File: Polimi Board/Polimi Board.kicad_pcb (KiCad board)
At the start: 2 copper layers, 96 parts, among them IC1 M95512-RMN6P, J1 I2C Oled Screen, J2 DM3AT-SF-PEJM5_40_, J3 65100516121, J4 UART Conn, J5 JTAG Conn, J7 65100516121, J8 7499010121A, SW1 MCU Reset, SW2 SW_Push, SW3 SW_Push, SW4 SW_Push, SW5 SW_Push, SW6 SW_Push, SW7 SW_Push, SW8 SW_Push, U1 STM32F205RCT6, U2 FT2232HL, U3 LAN8742A, U5 TLV76133DCY, Y1 ABL-25.000MHz-B1UB, Y2 ABL-12.000MHZ-20-D4HFI

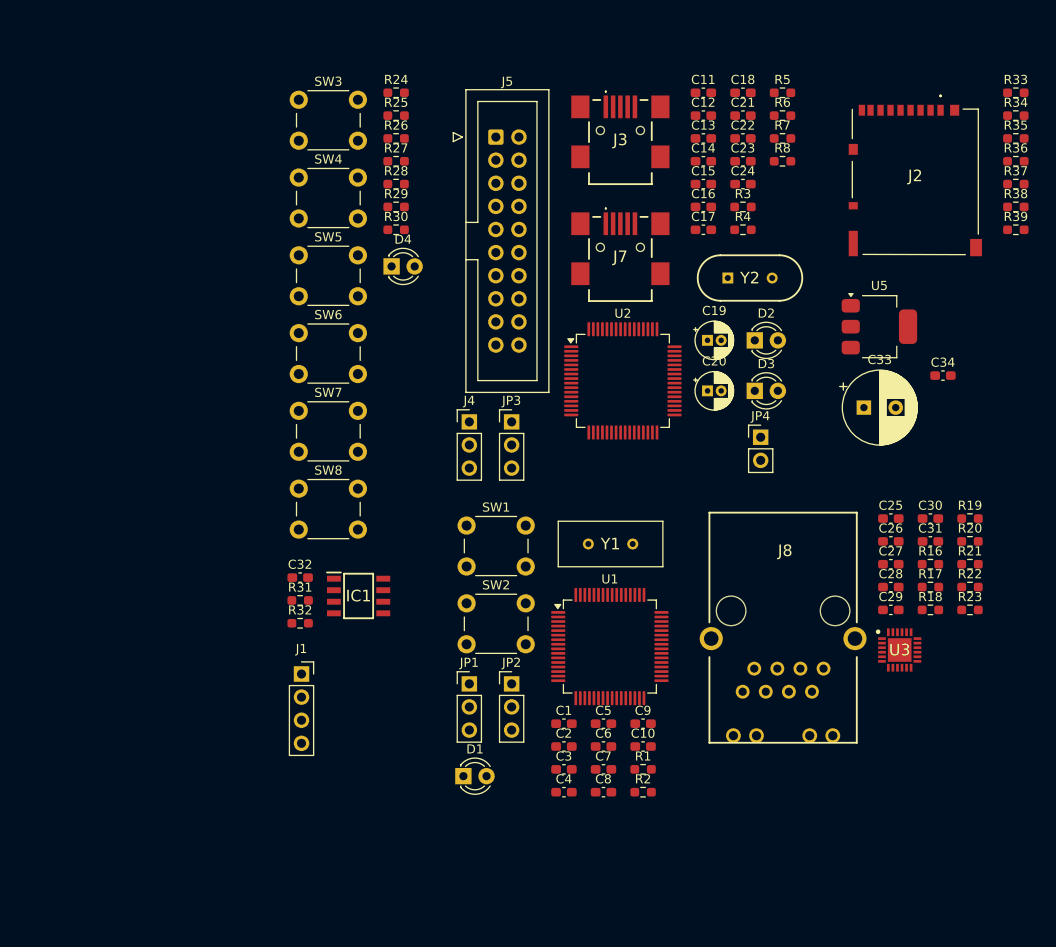
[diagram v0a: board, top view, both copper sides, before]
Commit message: PCB wip
before holidays
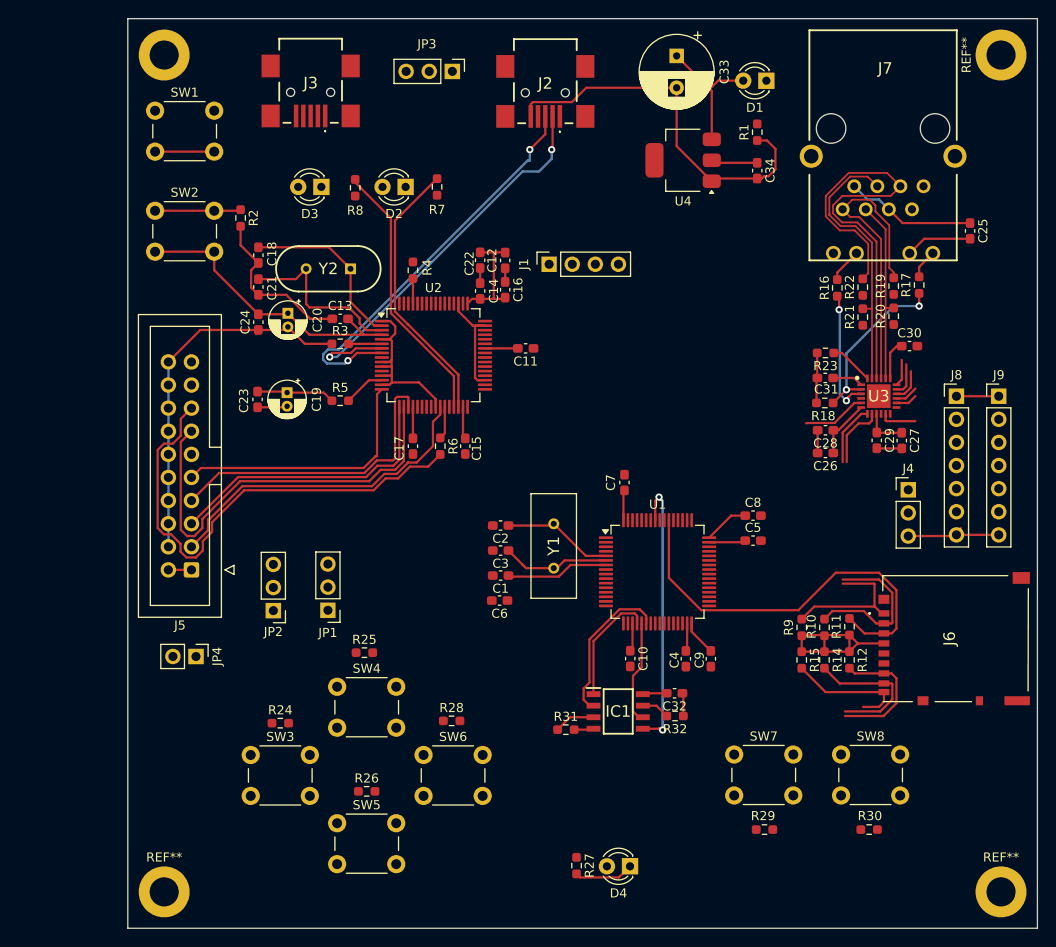
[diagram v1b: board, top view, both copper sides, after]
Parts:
- removed R33, R34, R35, R36, R37, R38, R39: 47k, Resistor_SMD:R_0603_1608Metric_Pad0.98x0.95mm_HandSolder
- removed U5: TLV76133DCY, Package_TO_SOT_SMD:SOT-223-3_TabPin2
- added J6: DM3AT-SF-PEJM5_40_, SamacSys_Parts:DM3ATSFPEJM540, F.Cu at (185.7, 106.4)
- added J9: Conn_01x07_Pin, Connector_PinHeader_2.54mm:PinHeader_1x07_P2.54mm_Vertical, F.Cu at (197.8, 82.5)
- added R10: 47k, Resistor_SMD:R_0603_1608Metric_Pad0.98x0.95mm_HandSolder, F.Cu at (178.6, 107.9)
- added R11: 47k, Resistor_SMD:R_0603_1608Metric_Pad0.98x0.95mm_HandSolder, F.Cu at (181.3, 107.8)
- added R12: 47k, Resistor_SMD:R_0603_1608Metric_Pad0.98x0.95mm_HandSolder, F.Cu at (181.3, 111.5)
- added R14: 47k, Resistor_SMD:R_0603_1608Metric_Pad0.98x0.95mm_HandSolder, F.Cu at (178.6, 111.5)
- added R15: 47k, Resistor_SMD:R_0603_1608Metric_Pad0.98x0.95mm_HandSolder, F.Cu at (176.1, 111.5)
- added R9: 47k, Resistor_SMD:R_0603_1608Metric_Pad0.98x0.95mm_HandSolder, F.Cu at (176.1, 107.9)
- added REF**: MountingHole_3.2mm_M3_DIN965_Pad, MountingHole:MountingHole_3.2mm_M3_DIN965_Pad, F.Cu at (106.0, 45.0)
- added REF**: MountingHole_3.2mm_M3_DIN965_Pad, MountingHole:MountingHole_3.2mm_M3_DIN965_Pad, F.Cu at (198.0, 45.0)
- added REF**: MountingHole_3.2mm_M3_DIN965_Pad, MountingHole:MountingHole_3.2mm_M3_DIN965_Pad, F.Cu at (198.0, 137.0)
- added REF**: MountingHole_3.2mm_M3_DIN965_Pad, MountingHole:MountingHole_3.2mm_M3_DIN965_Pad, F.Cu at (106.0, 137.0)
- added U4: TLV76133DCY, Package_TO_SOT_SMD:SOT-223-3_TabPin2, F.Cu at (163.1, 56.6)
- J2: value DM3AT-SF-PEJM5_40_ -> 65100516121; footprint SamacSys_Parts:DM3ATSFPEJM540 -> SamacSys_Parts:65100516121
- J7: value 65100516121 -> 7499010121A; footprint SamacSys_Parts:65100516121 -> SamacSys_Parts:WURTH-7499010121A
- J8: value 7499010121A -> Conn_01x07_Pin; footprint SamacSys_Parts:WURTH-7499010121A -> Connector_PinHeader_2.54mm:PinHeader_1x07_P2.54mm_Vertical
- SW2: value SW_Push -> Boot
- moved R30 84.0 mm to (183.5, 130.2), turned to 180 degrees
- moved D1 83.4 mm to (172.2, 47.8), turned to 180 degrees
- moved R27 79.9 mm to (151.3, 134.1), turned to -90 degrees
- moved R29 79.5 mm to (172.0, 130.2), turned to 180 degrees
- moved R2 77.1 mm to (114.4, 62.9), turned to -90 degrees
- moved SW3 72.2 mm to (115.5, 122.0)
- moved R26 71.9 mm to (128.3, 126.0)
- moved R1 71.2 mm to (171.2, 53.5), turned to 90 degrees
- moved D4 71.0 mm to (157.2, 134.2), turned to 180 degrees
- moved R24 70.5 mm to (118.8, 118.5)
- moved JP4 66.6 mm to (109.5, 111.1), turned to -90 degrees
- moved SW8 66.4 mm to (180.4, 121.9)
- moved SW5 62.6 mm to (125.0, 129.4)
- moved SW7 61.0 mm to (168.7, 121.9)
- moved C23 59.4 mm to (116.3, 82.9), turned to 90 degrees
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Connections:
- J2 pad 1: /SDMMC_D2 -> /USB Programming and OTP/VBUS_PROG
- J2 pad 2: /SDMMC_D3 -> Net-(U2-DM)
- J2 pad 3: /SDMMC_CMD -> Net-(U2-DP)
- J2 pad 4: +3.3V -> unconnected-(J2-Pad4)
- J2 pad 5: /SDMMC_CK -> GND
- J3 pad 1: /USB Programming and OTP/VBUS_PROG -> /USB Programming and OTP/VBUS_OTG
- J3 pad 2: Net-(U2-DM) -> /OTG_DM
- J3 pad 3: Net-(U2-DP) -> /OTG_DP
- J7 pad 1: /USB Programming and OTP/VBUS_OTG -> /Ethernet/TXP
- J7 pad 2: /OTG_DM -> +3V3
- J7 pad 3: /OTG_DP -> /Ethernet/TXN
- J7 pad 4: unconnected-(J7-Pad4) -> /Ethernet/RXP
- J7 pad 5: GND -> +3V3
- J8 pad 1: /Ethernet/TXP -> +3.3V
- J8 pad 2: +3V3 -> /GPIO_EXT_1
- J8 pad 3: /Ethernet/TXN -> /GPIO_EXT_2
- J8 pad 4: /Ethernet/RXP -> /GPIO_EXT_3
- J8 pad 5: +3V3 -> /GPIO_EXT_4
- J8 pad 6: /Ethernet/RXN -> /GPIO_EXT_5
- J8 pad 7: unconnected-(J8-Pad7) -> GND
- R16 pad 1: Net-(J8-Pad11) -> Net-(J7-Pad10)
- R16 pad 2: GND -> /Ethernet/LED1
- R17 pad 1: Net-(J8-Pad9) -> /Ethernet/LED2
- R17 pad 2: GND -> Net-(J7-Pad12)
- U1 pad 14: unconnected-(U1-PA0-Pad14) -> /GPIO_EXT_1
- U1 pad 16: unconnected-(U1-PA2-Pad16) -> /GPIO_EXT_2
- U1 pad 17: unconnected-(U1-PA3-Pad17) -> /GPIO_EXT_3
- U1 pad 26: unconnected-(U1-PB0-Pad26) -> /GPIO_EXT_4
- U1 pad 27: unconnected-(U1-PB1-Pad27) -> /GPIO_EXT_5
- U1 pad 28: unconnected-(U1-PB2-Pad28) -> /GPIO_EXT_6
- U1 pad 29: unconnected-(U1-PB10-Pad29) -> /GPIO_EXT_9
- U1 pad 38: /SDMMC_WP -> /GPIO_EXT_10
- U1 pad 61: unconnected-(U1-PB8-Pad61) -> /GPIO_EXT_7
- U1 pad 62: unconnected-(U1-PB9-Pad62) -> /GPIO_EXT_8
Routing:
- net GND: track 0.00 -> 171.4 mm
- net +3.3V: track 0.00 -> 103.0 mm
- net /USB Programming and OTP/JTAG_SRST: track 0.00 -> 54.1 mm
- net /Ethernet/RXN: track 0.00 -> 52.4 mm
- net /JTAG_TD0: track 0.00 -> 46.1 mm
- net /SDMMC_CMD: track 0.00 -> 45.6 mm
- net Net-(U2-DP): track 0.00 -> 45.0 mm, vias 0 -> 2
- net Net-(U2-DM): track 0.00 -> 44.7 mm, vias 0 -> 2
- net /JTAG_TRST: track 0.00 -> 36.5 mm
- net /Ethernet/TXP: track 0.00 -> 34.0 mm
- net /JTAG_TMS: track 0.00 -> 33.5 mm
- net /JTAG_TDI: track 0.00 -> 31.6 mm
- net /Flash_MOSI: track 0.00 -> 31.4 mm, vias 0 -> 2
- net /Ethernet/RXP: track 0.00 -> 30.6 mm
- net Net-(U2-ACBUS4): track 0.00 -> 29.9 mm
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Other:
- board outline added: 100 x 100 mm

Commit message: almost finish
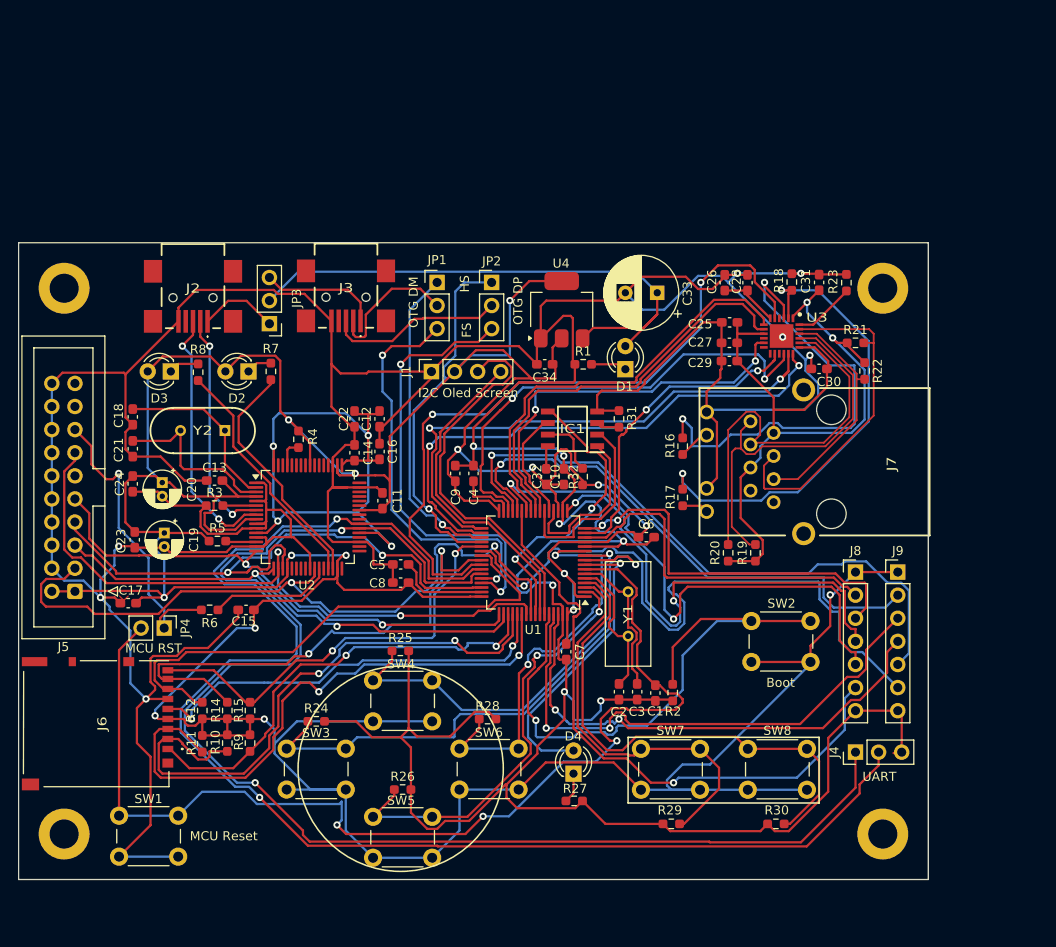
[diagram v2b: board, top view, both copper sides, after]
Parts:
- added G***: LOGO, graphics:Logo, B.Cu at (141.0, 98.6)
- J4: value UART Conn -> UART
- JP4: value MCU_RST -> MCU RST
- moved SW1 82.0 mm to (107.5, 133.1), turned to 180 degrees
- moved J6 81.3 mm to (105.8, 121.3), turned to -90 degrees
- moved SW2 79.6 mm to (170.6, 107.2)
- moved R11 72.3 mm to (110.2, 120.7), turned to -90 degrees
- moved R12 71.4 mm to (110.2, 117.1), turned to 90 degrees
- moved R2 70.6 mm to (161.9, 115.1)
- moved R10 66.9 mm to (112.9, 120.6), turned to -90 degrees
- moved R14 65.9 mm to (112.9, 117.1), turned to 90 degrees
- moved R9 62.0 mm to (115.4, 120.6), turned to -90 degrees
- moved R15 60.9 mm to (115.4, 117.1), turned to 90 degrees
- moved J2 44.8 mm to (109.2, 70.4)
- moved JP2 43.3 mm to (142.0, 70.0), turned to 0 degrees
- moved C8 39.4 mm to (132.0, 103.0), turned to 180 degrees
- moved C5 38.8 mm to (132.0, 101.0), turned to 180 degrees
- moved JP1 38.0 mm to (136.0, 70.0), turned to 0 degrees
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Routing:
- net GND: track 171.4 -> 675.1 mm, vias 0 -> 14
- net +3.3V: track 103.0 -> 521.0 mm, vias 0 -> 16
- net /USART_TX: track 0.00 -> 156.6 mm, vias 0 -> 2
- net /USART_RX: track 0.00 -> 153.5 mm, vias 0 -> 2
- net /MCU_RST: track 17.8 -> 122.3 mm, vias 0 -> 3
- net /GPIO_EXT_10: track 0.00 -> 71.7 mm, vias 0 -> 1
- net /MCO: track 6.96 -> 77.3 mm, vias 0 -> 2
- net /GPIO_EXT_9: track 0.00 -> 69.2 mm, vias 0 -> 1
- net /GPIO_EXT_5: track 0.00 -> 67.4 mm, vias 0 -> 1
- net /GPIO1: track 0.00 -> 62.7 mm, vias 0 -> 1
- net /GPIO_EXT_4: track 0.00 -> 61.7 mm, vias 0 -> 2
- net /GPIO_EXT_7: track 0.00 -> 59.6 mm, vias 0 -> 2
- net /GPIO_EXT_6: track 0.00 -> 59.1 mm, vias 0 -> 1
- net +3V3: track 27.0 -> 85.7 mm, vias 0 -> 2
- net Net-(U1-BOOT0): track 9.45 -> 67.1 mm, vias 0 -> 1
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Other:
- board size 100 x 100 mm -> 100 x 70 mm
- board text added: "FS"
- board text added: "HS"
- board text added: "OTG DM"
- board text added: "OTG DP"
